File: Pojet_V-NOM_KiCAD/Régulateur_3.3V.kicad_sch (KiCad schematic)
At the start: 3 parts

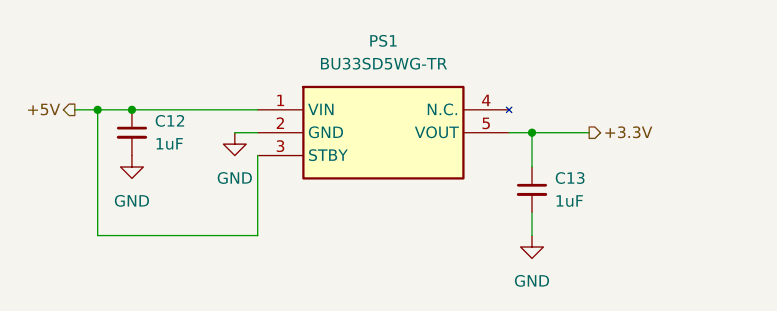
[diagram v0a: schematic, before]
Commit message: Maj
Maj lidar et regualteur
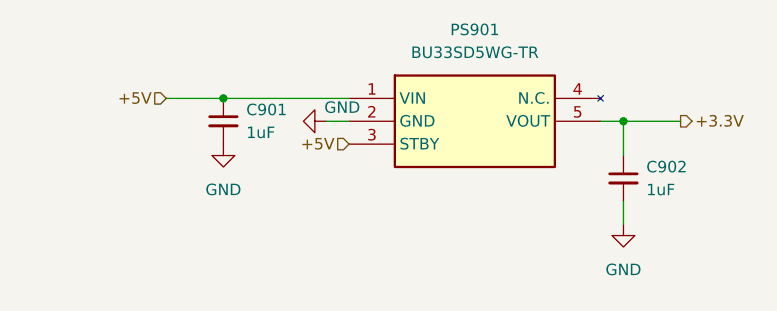
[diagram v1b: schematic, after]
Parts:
- removed C12, C13: 1uF, symbol Device:C_Small
- removed PS1: BU33SD5WG-TR, SOT95P280X125-5N, symbol BU33SD5WG-TR:BU33SD5WG-TR
- added C901, C902: 1uF, symbol Device:C_Small
- added PS901: BU33SD5WG-TR, SOT95P280X125-5N, symbol BU33SD5WG-TR:BU33SD5WG-TR
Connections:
- net +3.3V: now also C902.1, PS901.5 (VOUT)
- net +5V: now also C901.1, PS901.1 (VIN), PS901.3 (STBY)
- net GND: now also C901.2, C902.2, PS901.2 (GND)
